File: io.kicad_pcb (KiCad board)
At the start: 2 copper layers, 142 x 100 mm, 48 parts, among them CON1 AVR_ISP, IC1 ATMEGA644P-P, J1 DB9, J2 DB9, P1 CONN_CTL_DATA, P2 CONN_ADDR, P3 SLOT1, P4 SLOT2, P5 SLOT3, P6 CONN_01X02, P7 SLOT_EX_ADDR, U1 74LS138, U2 74HC245, U3 DISP_5110, U5 74HC05, U6 MAX232, Y1 14.7456M

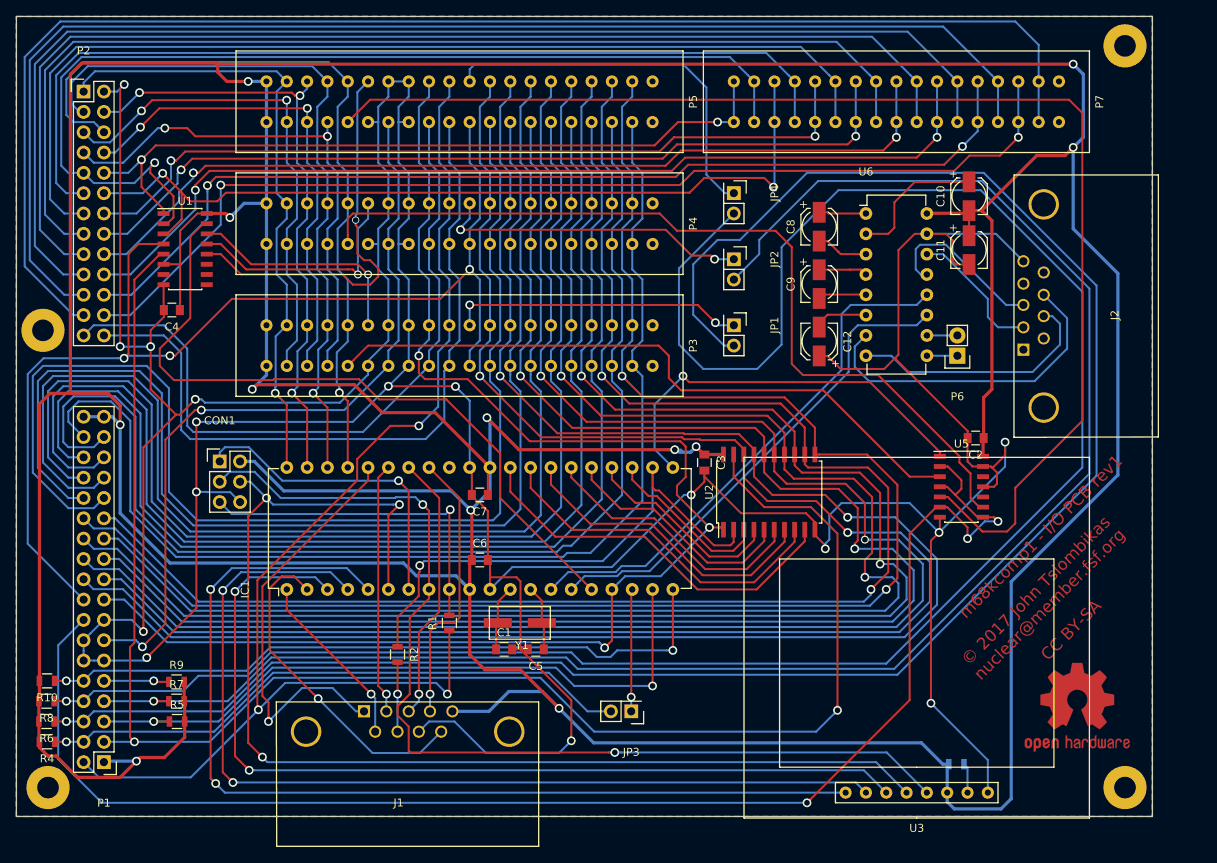
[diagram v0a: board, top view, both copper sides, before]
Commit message: io lite
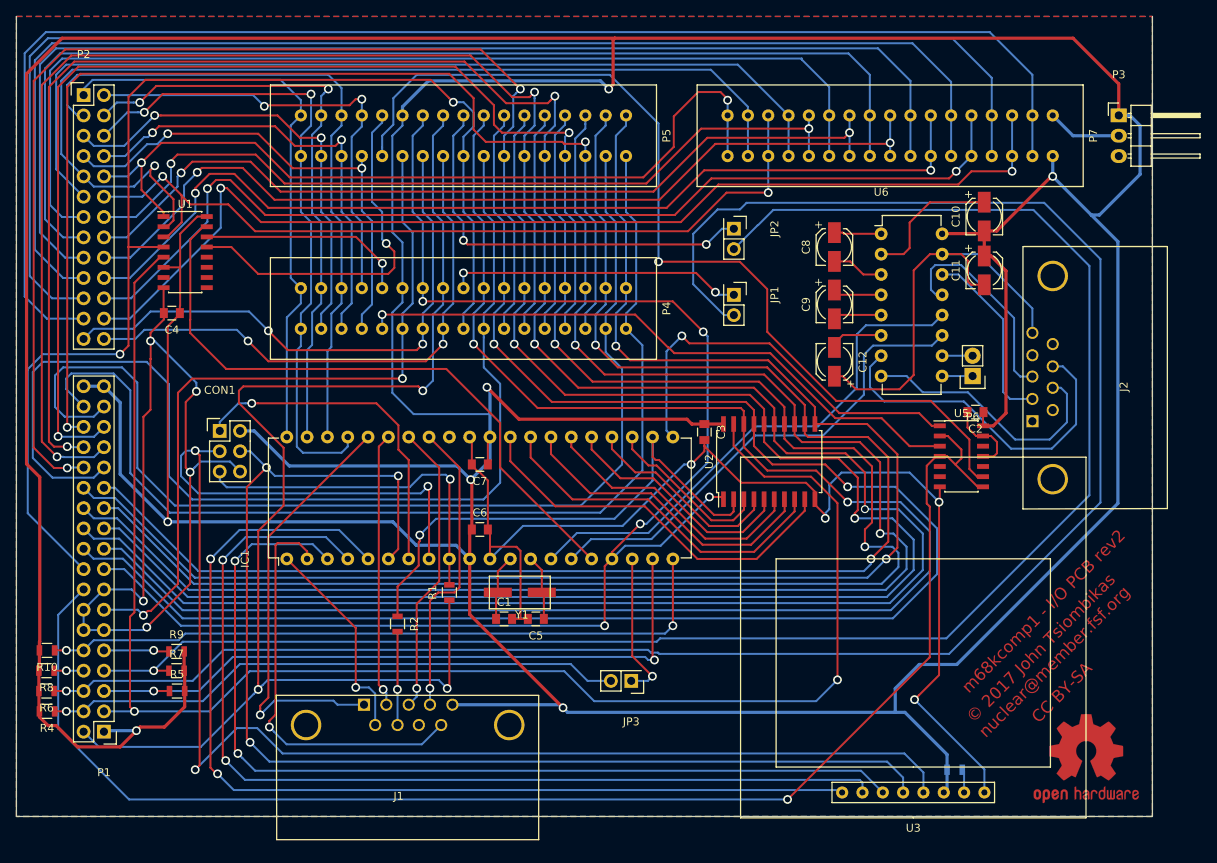
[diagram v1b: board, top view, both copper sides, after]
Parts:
- removed JP4: INT_S3, Pin_Headers:Pin_Header_Straight_2x01
- removed REF** (x4): MountingHole_2.7mm_M2.5_Pad, Mounting_Holes:MountingHole_2.7mm_M2.5_Pad
- P3: value SLOT1 -> SLOT_PWR; footprint m68kcomp1:edgecon_2x20 -> Pin_Headers:Pin_Header_Angled_1x03
- P4: value SLOT2 -> SLOT1; footprint m68kcomp1:edgecon_2x20 -> m68kcomp1:edgecon_2x17
- P5: value SLOT3 -> SLOT2; footprint m68kcomp1:edgecon_2x20 -> m68kcomp1:edgecon_2x17
- moved P3 87.3 mm to (172.6, 57.6), turned to 0 degrees
- moved P4 10.6 mm to (90.7, 81.7)
- moved J2 9.02 mm to (161.8, 95.8)
- moved REF*** 6.51 mm to (168.5, 138.0)
- moved P7 4.32 mm to (144.0, 60.1)
- moved P5 4.28 mm to (90.7, 60.1)
- moved R10 3.81 mm to (38.6, 124.5)
- moved C1 3.81 mm to (95.7, 120.5)
- moved C5 3.81 mm to (99.7, 120.5)
- moved C6 3.81 mm to (92.7, 109.3)
- moved C7 3.81 mm to (92.7, 101.2)
- moved IC1 3.81 mm to (68.6, 113.0)
- moved JP2 3.81 mm to (124.5, 71.8)
- moved JP3 3.81 mm to (111.6, 128.3)
- moved P1 3.81 mm to (45.7, 134.6)
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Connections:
- P3 pad 2: VCC -> GND
- P3 pad 3: /A5 -> GND
- P4 pad 1: VCC -> /A4
- P4 pad 10: /A4 -> /~EN_S1
- P4 pad 11: GND -> /CLK20
- P4 pad 12: /~EN_S2 -> VCC
- P4 pad 13: /CLK20 -> /~UDS
- P4 pad 14: GND -> /~WR
- P4 pad 15: GND -> /~LDS
- P4 pad 16: GND -> /~SYS_RESET
- P4 pad 17: /~UDS -> /~AS
- P4 pad 18: /~WR -> /~INTS1
- P4 pad 19: /~LDS -> /BUS8
- P4 pad 2: VCC -> /A1
- P4 pad 20: /~SYS_RESET -> /BUS0
- P4 pad 21: /~AS -> /BUS9
- P4 pad 22: /~INTS2 -> /BUS1
- P4 pad 23: /BUS8 -> /BUS10
- P4 pad 24: /BUS0 -> /BUS2
- P4 pad 25: /BUS9 -> /BUS11
- P4 pad 26: /BUS1 -> /BUS3
- P4 pad 27: /BUS10 -> /BUS12
- P4 pad 28: /BUS2 -> /BUS4
- P4 pad 29: /BUS11 -> /BUS13
- P4 pad 30: /BUS3 -> /BUS5
- P4 pad 31: /BUS12 -> /BUS14
- P4 pad 32: /BUS4 -> /BUS6
- P4 pad 33: /BUS13 -> /BUS15
- P4 pad 34: /BUS5 -> /BUS7
- P4 pad 4: /A1 -> /A2
- P4 pad 6: /A2 -> /A3
- P4 pad 8: /A3 -> GND
- P4 pad 9: Net-(P4-Pad9) -> /DTACK_S1
- P5 pad 1: VCC -> /A4
- P5 pad 10: /A4 -> /~EN_S2
- P5 pad 11: GND -> /CLK20
- P5 pad 12: /~EN_S3 -> VCC
- P5 pad 13: /CLK20 -> /~UDS
- P5 pad 14: GND -> /~WR
- P5 pad 15: GND -> /~LDS
- P5 pad 16: GND -> /~SYS_RESET
- P5 pad 17: /~UDS -> /~AS
- P5 pad 18: /~WR -> /~INTS2
- P5 pad 19: /~LDS -> /BUS8
- P5 pad 2: VCC -> /A1
- P5 pad 20: /~SYS_RESET -> /BUS0
- P5 pad 21: /~AS -> /BUS9
- P5 pad 22: /~INTS3 -> /BUS1
- P5 pad 23: /BUS8 -> /BUS10
- P5 pad 24: /BUS0 -> /BUS2
- P5 pad 25: /BUS9 -> /BUS11
- P5 pad 26: /BUS1 -> /BUS3
- P5 pad 27: /BUS10 -> /BUS12
- P5 pad 28: /BUS2 -> /BUS4
- P5 pad 29: /BUS11 -> /BUS13
- P5 pad 30: /BUS3 -> /BUS5
- P5 pad 31: /BUS12 -> /BUS14
- P5 pad 32: /BUS4 -> /BUS6
- P5 pad 33: /BUS13 -> /BUS15
- P5 pad 34: /BUS5 -> /BUS7
- P5 pad 4: /A1 -> /A2
- P5 pad 6: /A2 -> /A3
- P5 pad 8: /A3 -> GND
- P5 pad 9: Net-(P5-Pad9) -> /DTACK_S2
- P7 pad 33: (no net) -> VCC
- P7 pad 34: (no net) -> GND
- U1 pad 12: /~EN_S3 -> (no net)
- U5 pad 3: Net-(P3-Pad9) -> /DTACK_S1
- U5 pad 5: Net-(P5-Pad9) -> (no net)
- U5 pad 6: /~DTACK -> (no net)
- U5 pad 9: Net-(P4-Pad9) -> /DTACK_S2
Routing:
- net /~IRQ5: track 256.3 -> 3.69 mm
- net GND: track 577.0 -> 388.4 mm, vias 16 -> 11
- net Net-(P5-Pad9): track 160.1 -> 0.00 mm
- net /DTACK_S2: track 0.00 -> 119.4 mm, vias 0 -> 1
- net Net-(P4-Pad9): track 108.9 -> 0.00 mm
- net Net-(P3-Pad9): track 83.5 -> 0.00 mm
- net /DTACK_S1: track 0.00 -> 78.3 mm, vias 0 -> 1
- net /SCK: track 127.9 -> 187.3 mm, vias 2 -> 3
- net /~EN_S3: track 50.1 -> 0.00 mm, vias 1 -> 0
- net /~INTS3: track 47.9 -> 0.00 mm
- net /~LDS: track 94.2 -> 69.9 mm, vias 0 -> 2
- net /~UDS: track 90.9 -> 70.7 mm, vias 0 -> 2
- net /A4: track 98.6 -> 82.1 mm, vias 1 -> 2
- net /~EN_S2: track 29.9 -> 45.9 mm
- net /BUS8: track 149.7 -> 137.6 mm
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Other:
- board text added: "m68kcomp1 - I/O PCB rev2"
- board text removed: "m68kcomp1 - I/O PCB rev1"
